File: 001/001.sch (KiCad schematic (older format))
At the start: 6 parts, among them U1 MF-Jalisco, U2 Firma, U3 PinBase

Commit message: Update battery holder
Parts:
- BT1: footprint MF-Jalisco:WA-BCMC -> MF-Jalisco:CR1220-Jalisco
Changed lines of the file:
@@
 F 0 "BT1" V 5800 2850 50  0000 C CNN
 F 1 "Battery_3V_Coin" V 5875 2850 50  0000 C CNN
-F 2 "MF-Jalisco:WA-BCMC" V 5525 2910 50  0001 C CNN
+F 2 "MF-Jalisco:CR1220-Jalisco" V 5525 2910 50  0001 C CNN
 F 3 "~" V 5525 2910 50  0001 C CNN
 	1    5525 2850

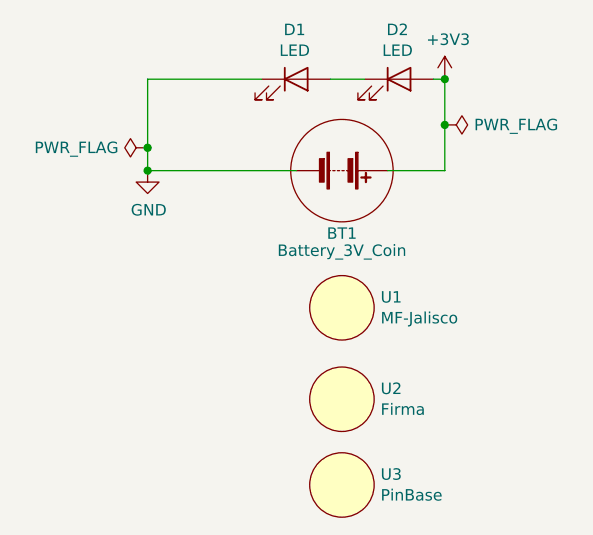
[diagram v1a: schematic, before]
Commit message: Changes
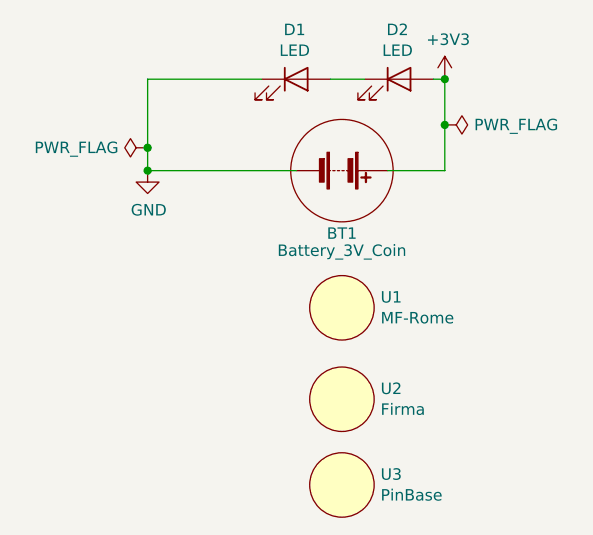
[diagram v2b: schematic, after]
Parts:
- BT1: footprint MF-Jalisco:CR1220-Jalisco -> MF-ROME:S8211R
- D1, D2: footprint MF-Jalisco:LED_D5.0mm_FlatTop -> MF-ROME:LED_D5.0mm_FlatTop
- U1: value MF-Jalisco -> MF-Rome; footprint MF-Jalisco:MF-Jalisco_50mm -> MF-ROME:Rome_100mm_01
- U2: footprint MF-Jalisco:firma_Cu_Mask -> MF-ROME:firma_Cu_Mask
- U3: footprint MF-Jalisco:PinBase -> MF-ROME:PinBase
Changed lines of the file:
@@
 F 0 "D1" H 5318 2666 50  0000 C CNN
 F 1 "LED" H 5318 2575 50  0000 C CNN
-F 2 "MF-Jalisco:LED_D5.0mm_FlatTop" H 5325 2450 50  0001 C CNN
+F 2 "MF-ROME:LED_D5.0mm_FlatTop" H 5325 2450 50  0001 C CNN
 F 3 "~" H 5325 2450 50  0001 C CNN
 	1    5325 2450
@@
 F 0 "D2" H 5768 2666 50  0000 C CNN
 F 1 "LED" H 5768 2575 50  0000 C CNN
-F 2 "MF-Jalisco:LED_D5.0mm_FlatTop" H 5775 2450 50  0001 C CNN
+F 2 "MF-ROME:LED_D5.0mm_FlatTop" H 5775 2450 50  0001 C CNN
 F 3 "~" H 5775 2450 50  0001 C CNN
 	1    5775 2450
@@
 P 5525 3450
 F 0 "U1" H 5694 3496 50  0000 L CNN
-F 1 "MF-Jalisco" H 5694 3405 50  0000 L CNN
-F 2 "MF-Jalisco:MF-Jalisco_50mm" H 5525 3450 50  0001 C CNN
+F 1 "MF-Rome" H 5694 3405 50  0000 L CNN
+F 2 "MF-ROME:Rome_100mm_01" H 5525 3450 50  0001 C CNN
 F 3 "" H 5525 3450 50  0001 C CNN
 	1    5525 3450
@@
 F 0 "BT1" V 5800 2850 50  0000 C CNN
 F 1 "Battery_3V_Coin" V 5875 2850 50  0000 C CNN
-F 2 "MF-Jalisco:CR1220-Jalisco" V 5525 2910 50  0001 C CNN
+F 2 "MF-ROME:S8211R" V 5525 2910 50  0001 C CNN
 F 3 "~" V 5525 2910 50  0001 C CNN
 	1    5525 2850
@@
 F 0 "U2" H 5694 3896 50  0000 L CNN
 F 1 "Firma" H 5694 3805 50  0000 L CNN
-F 2 "MF-Jalisco:firma_Cu_Mask" H 5525 3850 50  0001 C CNN
+F 2 "MF-ROME:firma_Cu_Mask" H 5525 3850 50  0001 C CNN
 F 3 "" H 5525 3850 50  0001 C CNN
 	1    5525 3850
@@
 F 0 "U3" H 5694 4271 50  0000 L CNN
 F 1 "PinBase" H 5694 4180 50  0000 L CNN
-F 2 "MF-Jalisco:PinBase" H 5525 4225 50  0001 C CNN
+F 2 "MF-ROME:PinBase" H 5525 4225 50  0001 C CNN
 F 3 "" H 5525 4225 50  0001 C CNN
 	1    5525 4225

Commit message: Fix Push
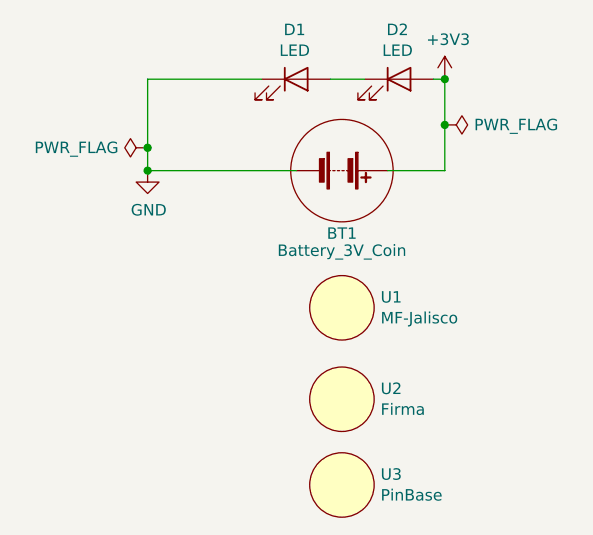
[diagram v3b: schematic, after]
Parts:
- BT1: footprint MF-ROME:S8211R -> MF-Jalisco:CR1220-Jalisco
- D1, D2: footprint MF-ROME:LED_D5.0mm_FlatTop -> MF-Jalisco:LED_D5.0mm_FlatTop
- U1: value MF-Rome -> MF-Jalisco; footprint MF-ROME:Rome_100mm_01 -> MF-Jalisco:MF-Jalisco_50mm
- U2: footprint MF-ROME:firma_Cu_Mask -> MF-Jalisco:firma_Cu_Mask
- U3: footprint MF-ROME:PinBase -> MF-Jalisco:PinBase
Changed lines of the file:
@@
 F 0 "D1" H 5318 2666 50  0000 C CNN
 F 1 "LED" H 5318 2575 50  0000 C CNN
-F 2 "MF-ROME:LED_D5.0mm_FlatTop" H 5325 2450 50  0001 C CNN
+F 2 "MF-Jalisco:LED_D5.0mm_FlatTop" H 5325 2450 50  0001 C CNN
 F 3 "~" H 5325 2450 50  0001 C CNN
 	1    5325 2450
@@
 F 0 "D2" H 5768 2666 50  0000 C CNN
 F 1 "LED" H 5768 2575 50  0000 C CNN
-F 2 "MF-ROME:LED_D5.0mm_FlatTop" H 5775 2450 50  0001 C CNN
+F 2 "MF-Jalisco:LED_D5.0mm_FlatTop" H 5775 2450 50  0001 C CNN
 F 3 "~" H 5775 2450 50  0001 C CNN
 	1    5775 2450
@@
 P 5525 3450
 F 0 "U1" H 5694 3496 50  0000 L CNN
-F 1 "MF-Rome" H 5694 3405 50  0000 L CNN
-F 2 "MF-ROME:Rome_100mm_01" H 5525 3450 50  0001 C CNN
+F 1 "MF-Jalisco" H 5694 3405 50  0000 L CNN
+F 2 "MF-Jalisco:MF-Jalisco_50mm" H 5525 3450 50  0001 C CNN
 F 3 "" H 5525 3450 50  0001 C CNN
 	1    5525 3450
@@
 F 0 "BT1" V 5800 2850 50  0000 C CNN
 F 1 "Battery_3V_Coin" V 5875 2850 50  0000 C CNN
-F 2 "MF-ROME:S8211R" V 5525 2910 50  0001 C CNN
+F 2 "MF-Jalisco:CR1220-Jalisco" V 5525 2910 50  0001 C CNN
 F 3 "~" V 5525 2910 50  0001 C CNN
 	1    5525 2850
@@
 F 0 "U2" H 5694 3896 50  0000 L CNN
 F 1 "Firma" H 5694 3805 50  0000 L CNN
-F 2 "MF-ROME:firma_Cu_Mask" H 5525 3850 50  0001 C CNN
+F 2 "MF-Jalisco:firma_Cu_Mask" H 5525 3850 50  0001 C CNN
 F 3 "" H 5525 3850 50  0001 C CNN
 	1    5525 3850
@@
 F 0 "U3" H 5694 4271 50  0000 L CNN
 F 1 "PinBase" H 5694 4180 50  0000 L CNN
-F 2 "MF-ROME:PinBase" H 5525 4225 50  0001 C CNN
+F 2 "MF-Jalisco:PinBase" H 5525 4225 50  0001 C CNN
 F 3 "" H 5525 4225 50  0001 C CNN
 	1    5525 4225
